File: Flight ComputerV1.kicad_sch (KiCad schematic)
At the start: 28 parts, among them J101 ICSP, J102 Screw_Terminal_01x02, J103 Conn_01x08, J104 Conn_01x07, J105 Micro_SD_Card, J106 Conn_02x10_Top_Bottom, SW101 1-1825910-8, U101 ATmega328PB-A, U102 LMT84DCK

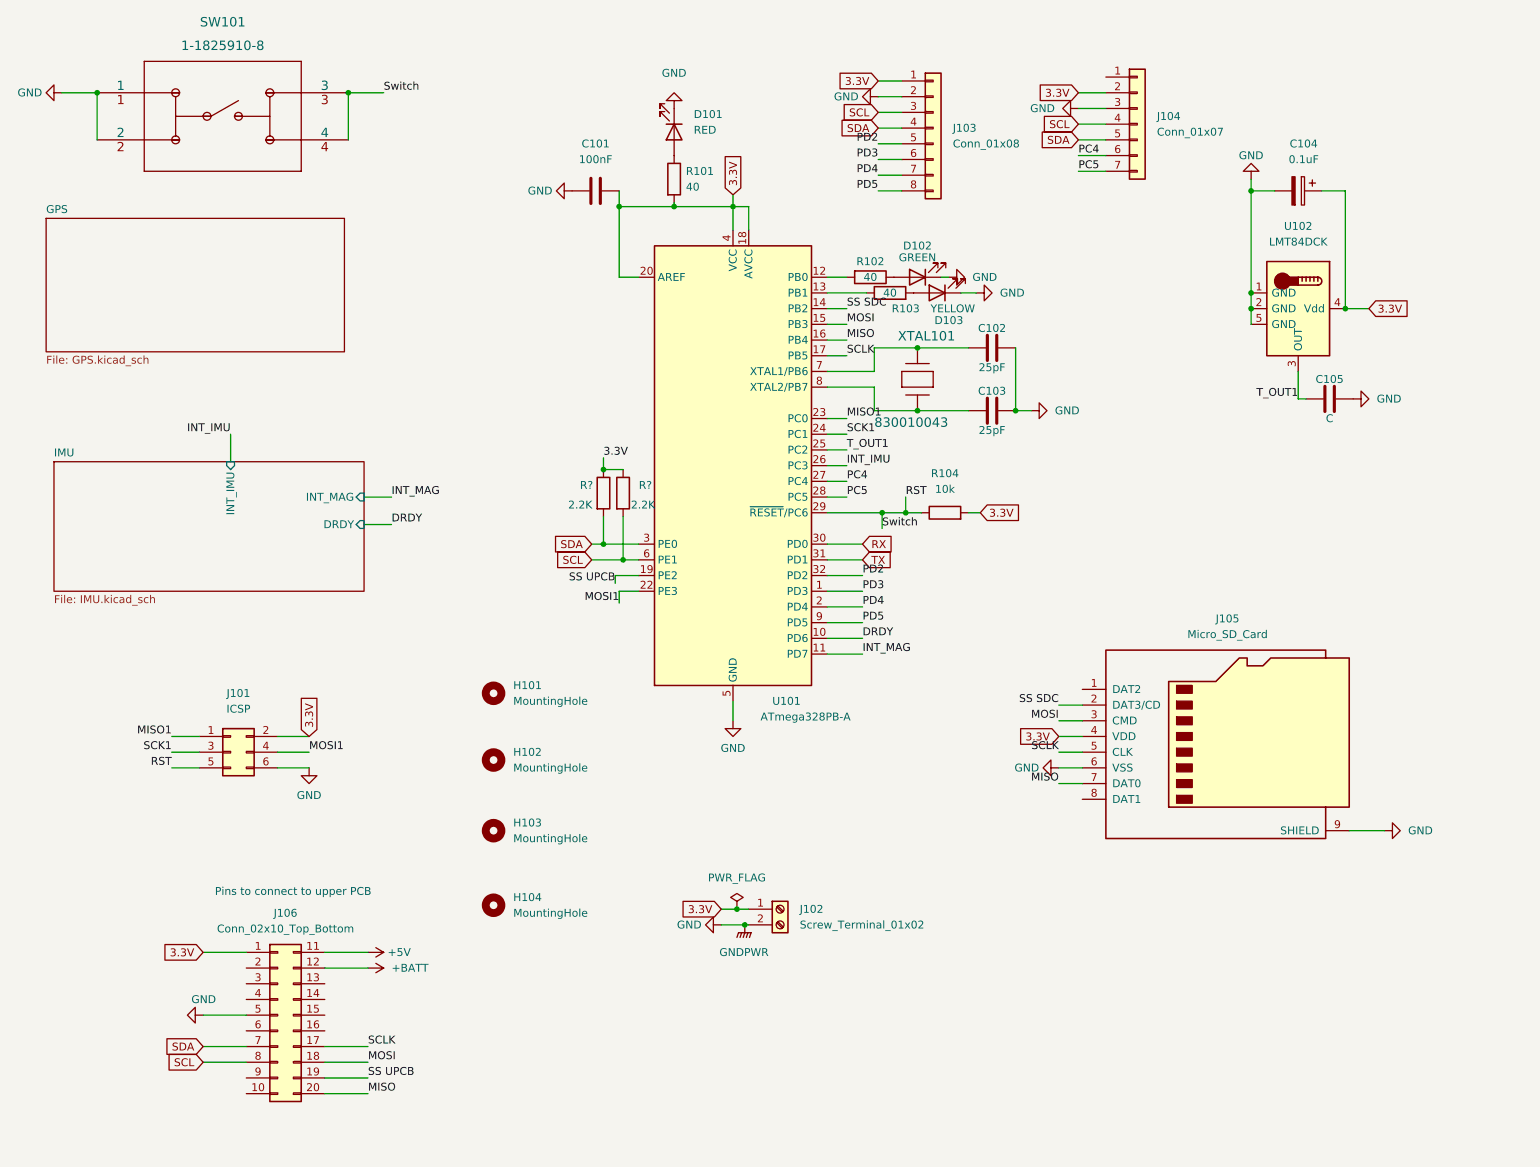
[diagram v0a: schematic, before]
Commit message: updates to schematics
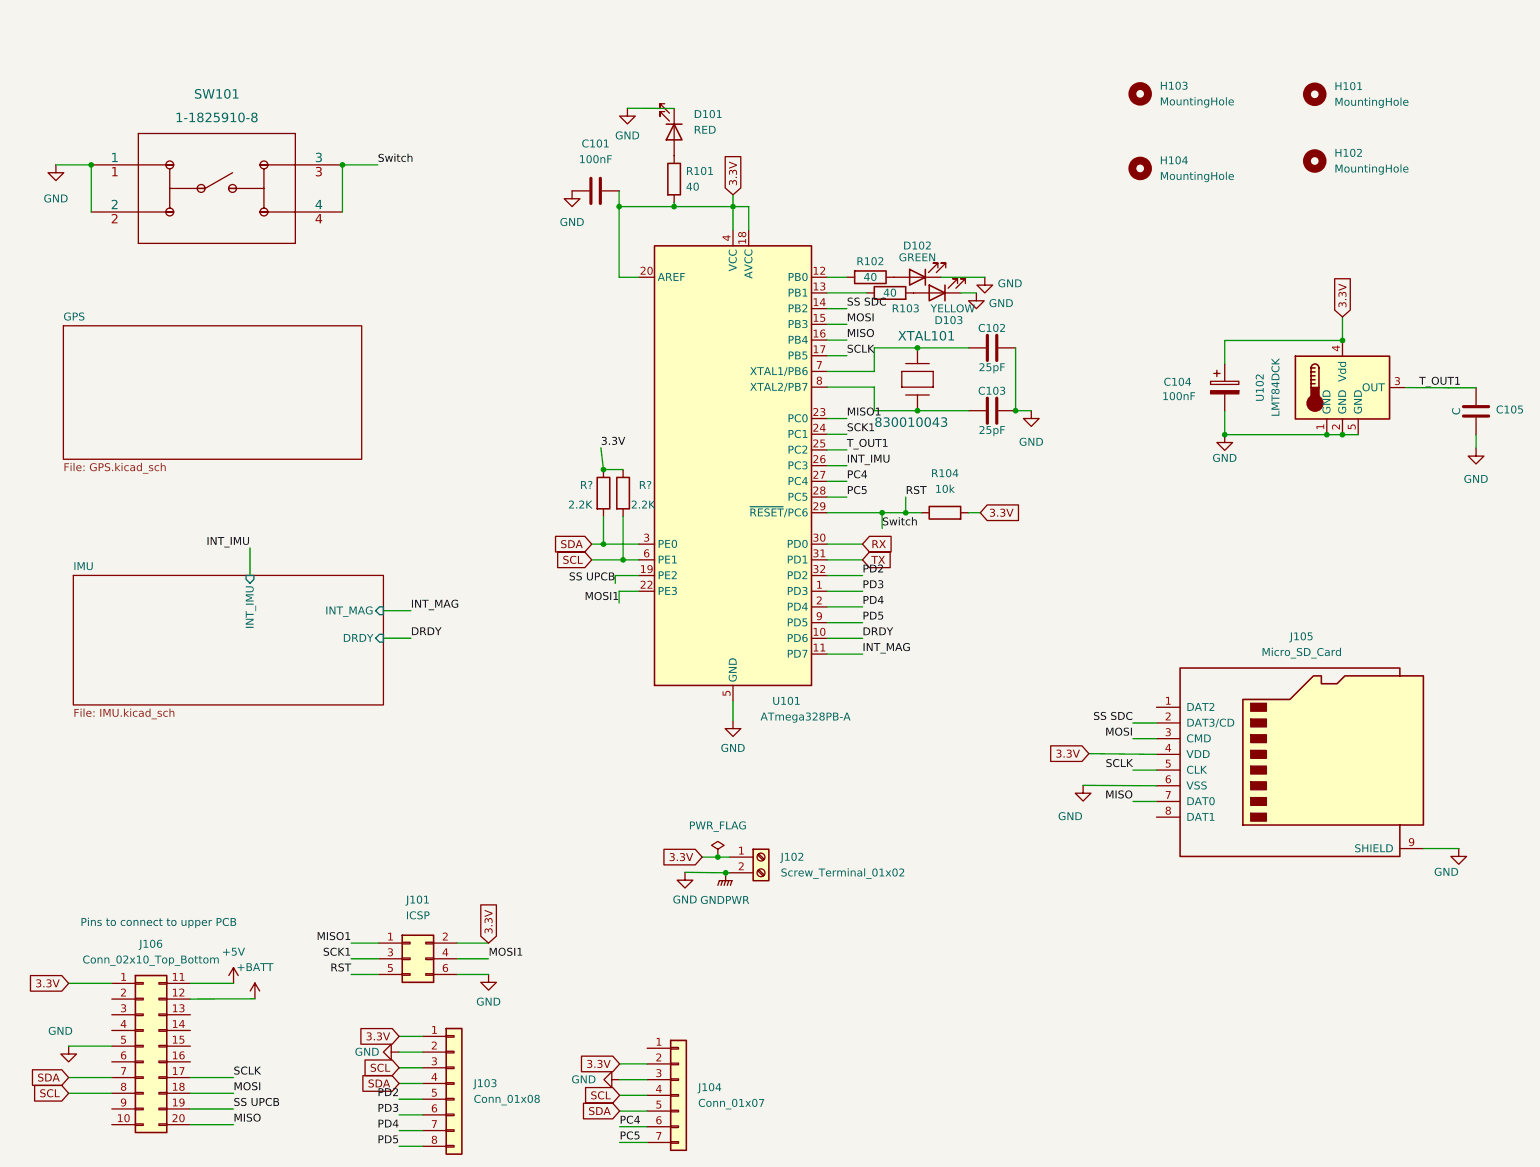
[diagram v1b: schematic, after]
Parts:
- C104: value 0.1uF -> 100nF
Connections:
- net T_OUT1: no longer C105.1, U102.3 (OUT)
- new net: C105.1, U102.3 (OUT)
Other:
- moved on the sheet: C104, C105, H101, H102, H103, H104, J101, J102, J103, J104, J105, J106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
